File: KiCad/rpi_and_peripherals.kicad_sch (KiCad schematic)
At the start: 6 parts, among them U3 LT1054, U4 PCM1808-Q1_PW_14, U9 PCM5102APW

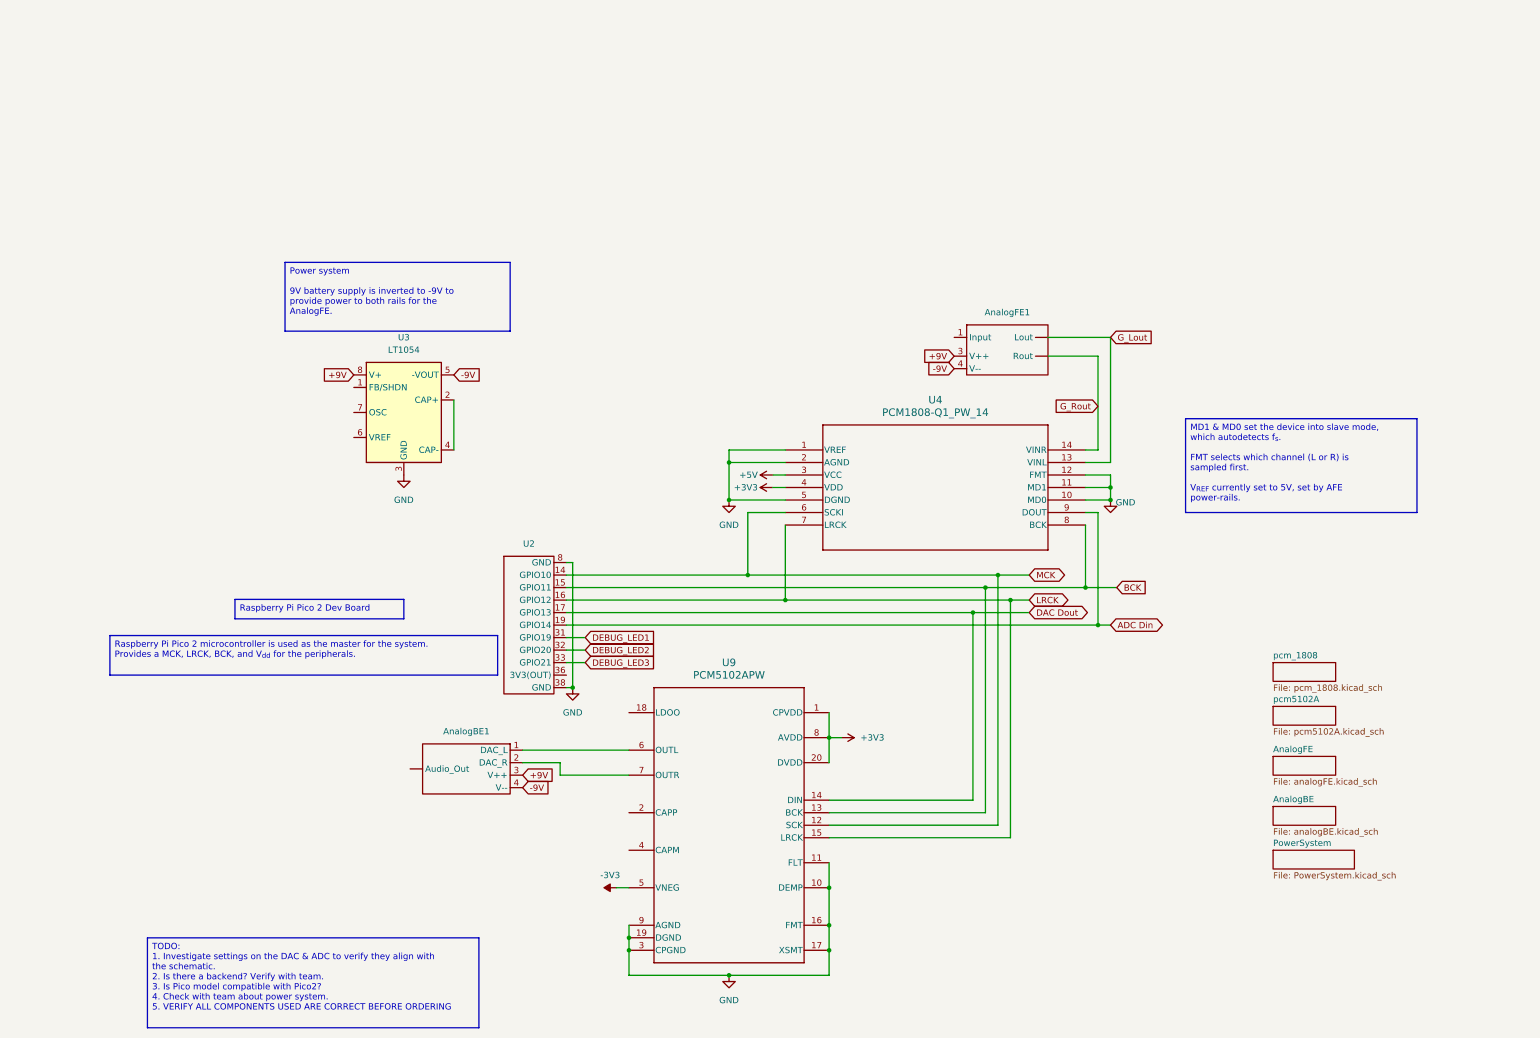
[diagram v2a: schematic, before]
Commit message: Updates for 10_18_26
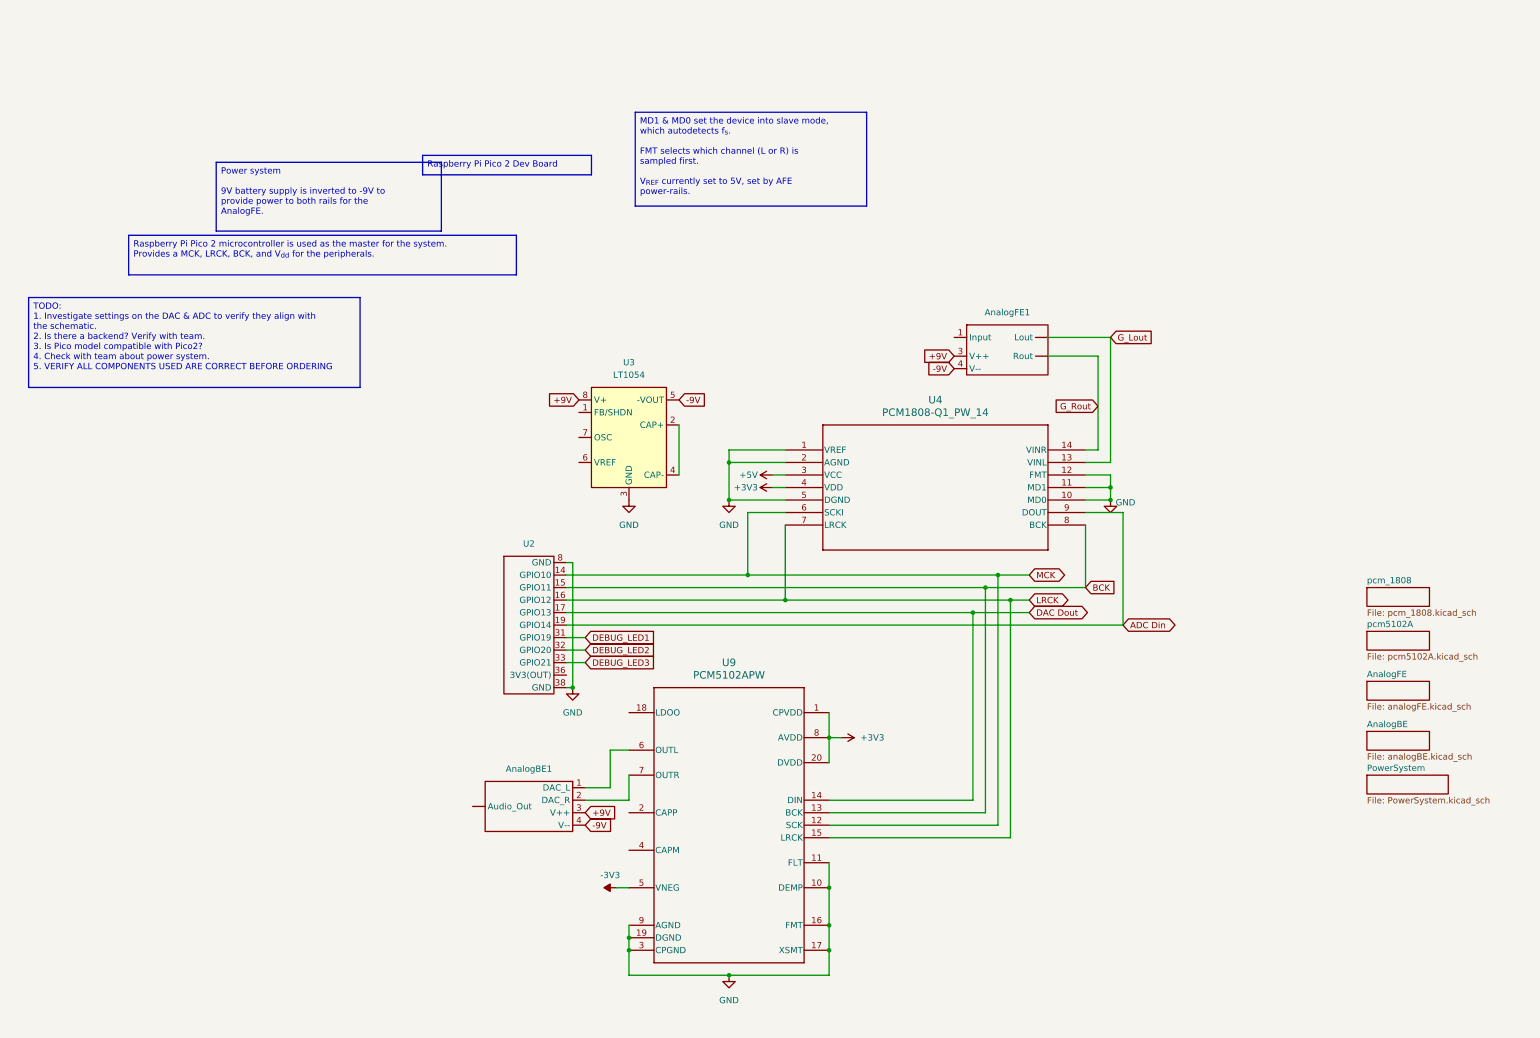
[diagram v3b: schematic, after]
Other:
- moved on the sheet: AnalogBE1, U3

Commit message: Pushing PCB, and controls schem
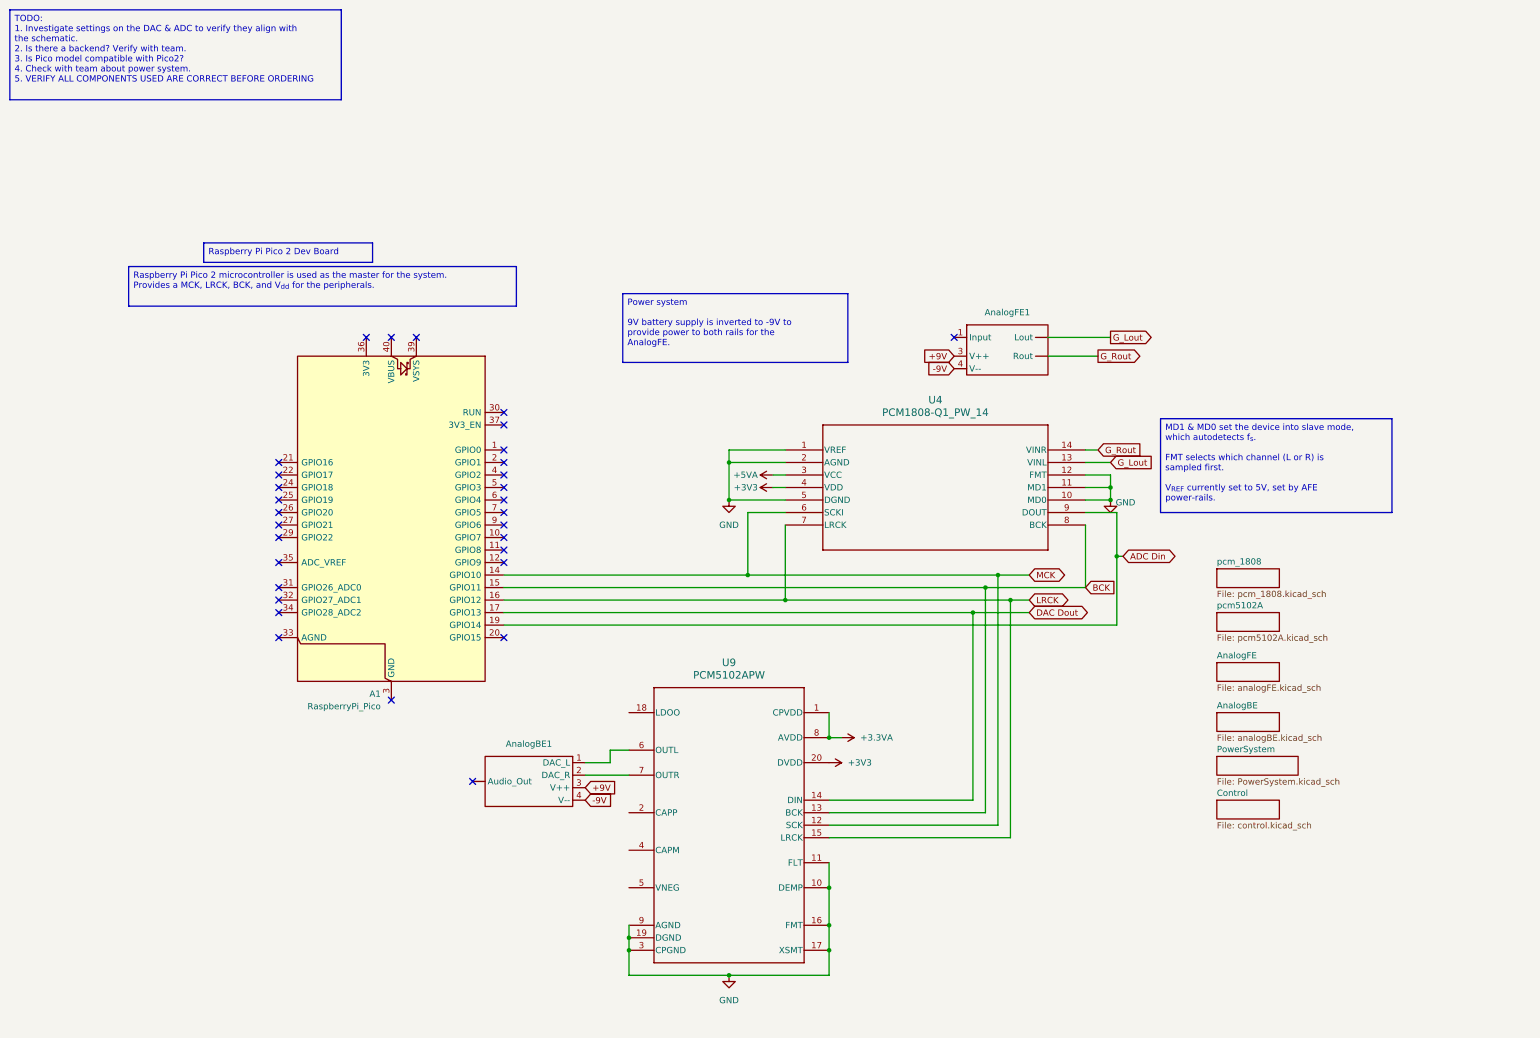
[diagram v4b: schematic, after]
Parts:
- removed U2: (no value), rpi_foot:rpi_dev_foot, symbol PCM1808:Pico_Dev_Board
- removed U3: LT1054, charge_pump:SOIC127P1030X265-16N, symbol Regulator_SwitchedCapacitor:LT1054
- added A1: RaspberryPi_Pico, Module:RaspberryPi_Pico_Common_Unspecified, symbol MCU_Module:RaspberryPi_Pico
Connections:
- net +3V3: no longer U9.1 (CPVDD), U9.8 (AVDD)
- net ADC Din: now also A1.19 (GPIO14)
- net BCK: now also A1.15 (GPIO11)
- net DAC Dout: now also A1.17 (GPIO13)
- net LRCK: now also A1.16 (GPIO12)
- net MCK: now also A1.14 (GPIO10)
- net +5V renamed +5VA
- net -3V3: no longer names the net of U9.5 (VNEG)
- new net: A1.13 (GND), A1.18 (GND), A1.23 (GND), A1.28 (GND), A1.3 (GND), A1.38 (GND), A1.8 (GND)
- new net +3.3VA: U9.1 (CPVDD), U9.8 (AVDD)
- no-connect marks 0 -> 31
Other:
- added sheet Control (control.kicad_sch)
- moved on the sheet: AnalogBE1
